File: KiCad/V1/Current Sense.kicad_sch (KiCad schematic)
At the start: 2 parts, among them U2 ${SIM.PARAMS}

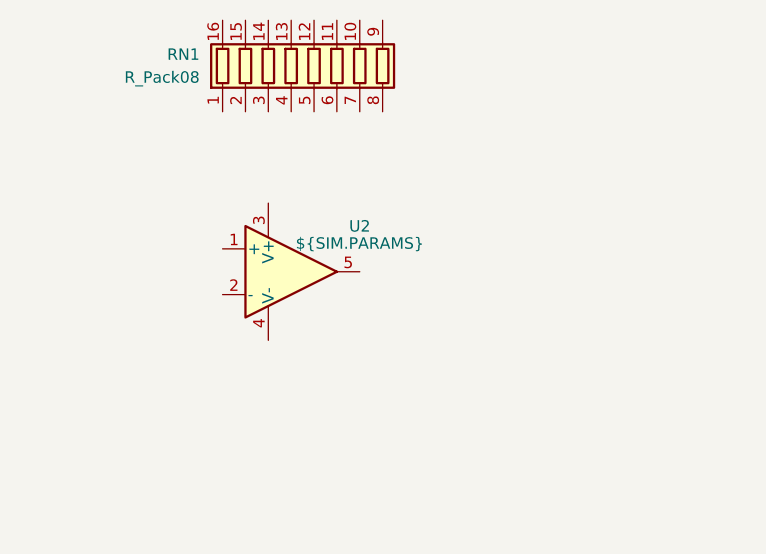
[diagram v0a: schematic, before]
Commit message: kicad scematic
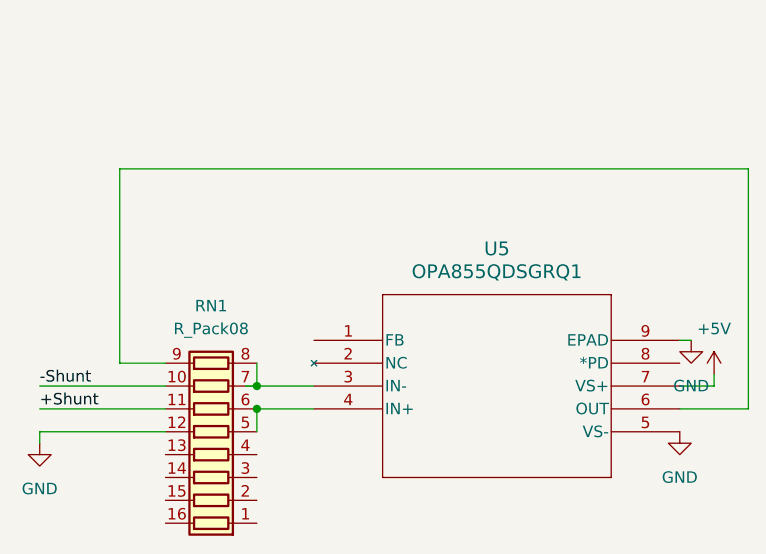
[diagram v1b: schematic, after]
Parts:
- removed U2: ${SIM.PARAMS}, symbol Simulation_SPICE:OPAMP
- added U5: OPA855QDSGRQ1, WSON8_DSG_TEX, symbol 2024-11-17_18-04-17:OPA855QDSGRQ1
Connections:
- net -Shunt: now reaches RN1.10 (R7.2)
- net +Shunt: now reaches RN1.11 (R6.2)
- net GND: now reaches RN1.12 (R5.2)
- net GND: now also U5.5 (VS-), U5.9 (EPAD)
- net at RN1.5 (R5.1): now also RN1.6 (R6.1), U5.4 (IN+)
- net at RN1.7 (R7.1): now also RN1.8 (R8.1), U5.3 (IN-)
- net at RN1.9 (R8.2): now also U5.6 (OUT)
- new net +5V: U5.7 (VS+)
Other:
- moved on the sheet: RN1
